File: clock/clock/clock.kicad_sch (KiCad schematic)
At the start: 44 parts, among them J1 AVR-ISP-6, J10 Conn_01x07_Male, J11 CV_IN, J12 CLOCK_OUT, J13 SUBDIV_OUT, J2 EURORACK_CONN_10, J3 Conn_01x05_Female, J4 Conn_01x05_Male, J5 Conn_01x05_Female, J6 Conn_01x05_Male, J7 Conn_01x05_Female, J8 Conn_01x05_Male, J9 Conn_01x07_Female, SW1 SW_Push, SW2 SW_Push, SW3 Rotary_Encoder_Switch, U1 ATmega328P-PU, U2 L7805, U3 SM460281N, U4 SM460281N, U5 SM460281N, Y1 16MHz

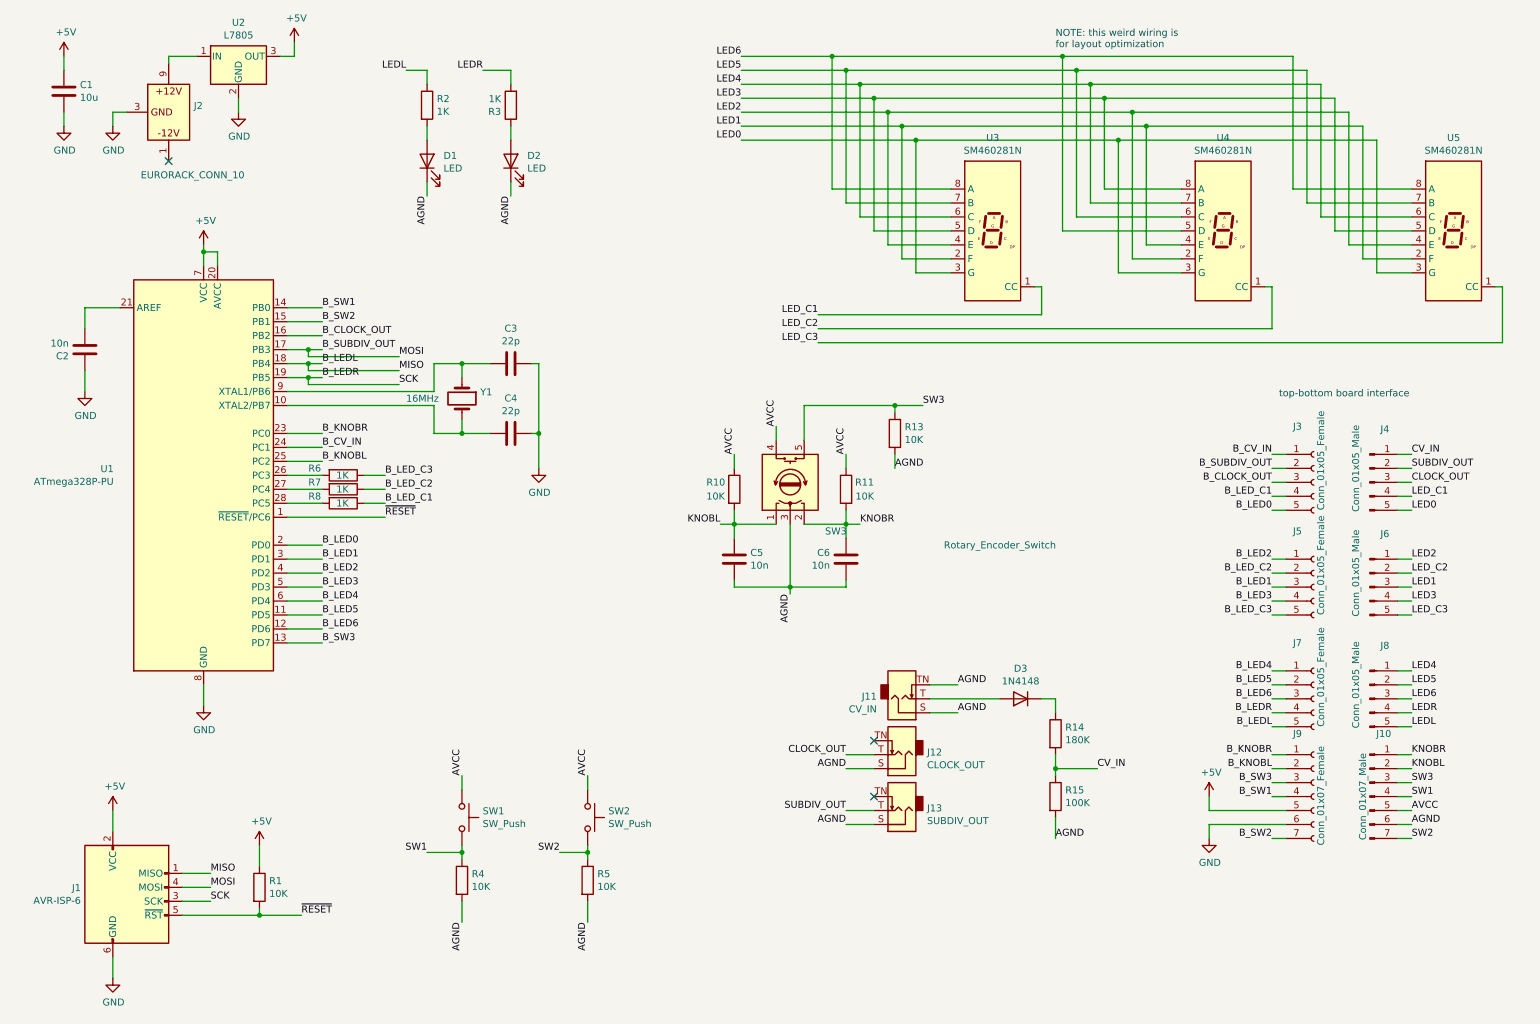
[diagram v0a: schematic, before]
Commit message: re-annotate schematic
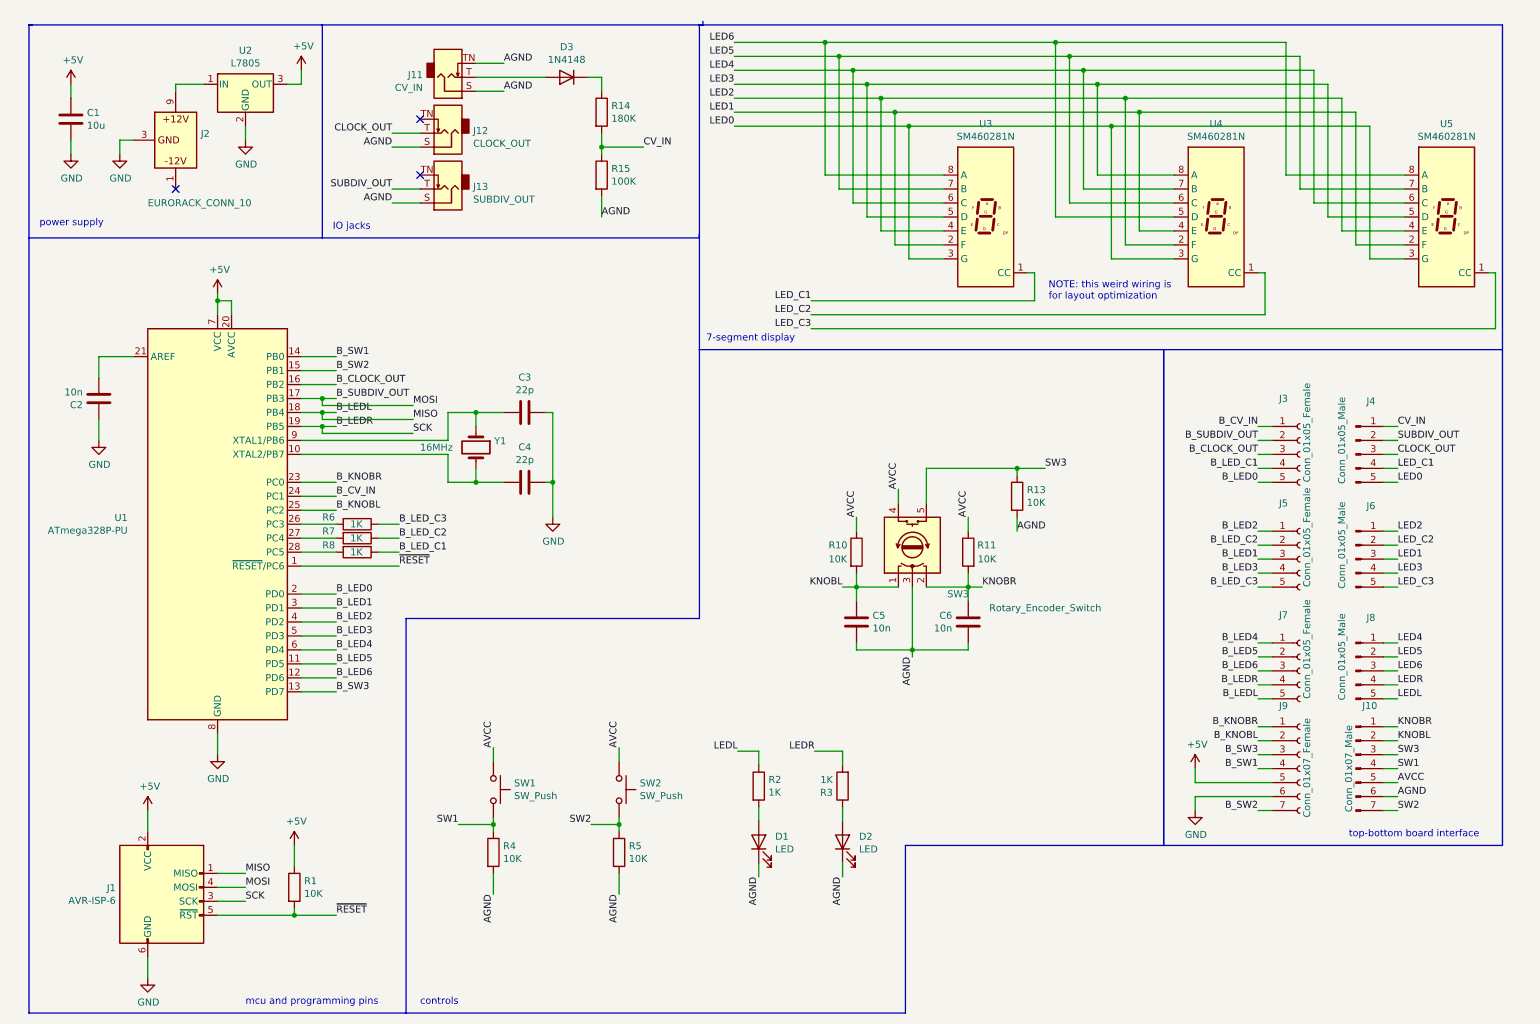
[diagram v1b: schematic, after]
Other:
- note added: "7-segment display"
- note added: "IO jacks"
- note added: "controls"
- note added: "mcu and programming pins"
- note added: "power supply"
- company: (none) -> rabid.audio
- title: (none) -> CLK
- moved on the sheet: C1, C2, C3, C4, C5, C6, D1, D2, D3, J1, J10, J11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
